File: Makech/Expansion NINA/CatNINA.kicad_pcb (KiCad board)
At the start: 2 copper layers, 22.9 x 30.9 mm, 10 parts, among them J1 ESP, U1 ESP32-WROOM

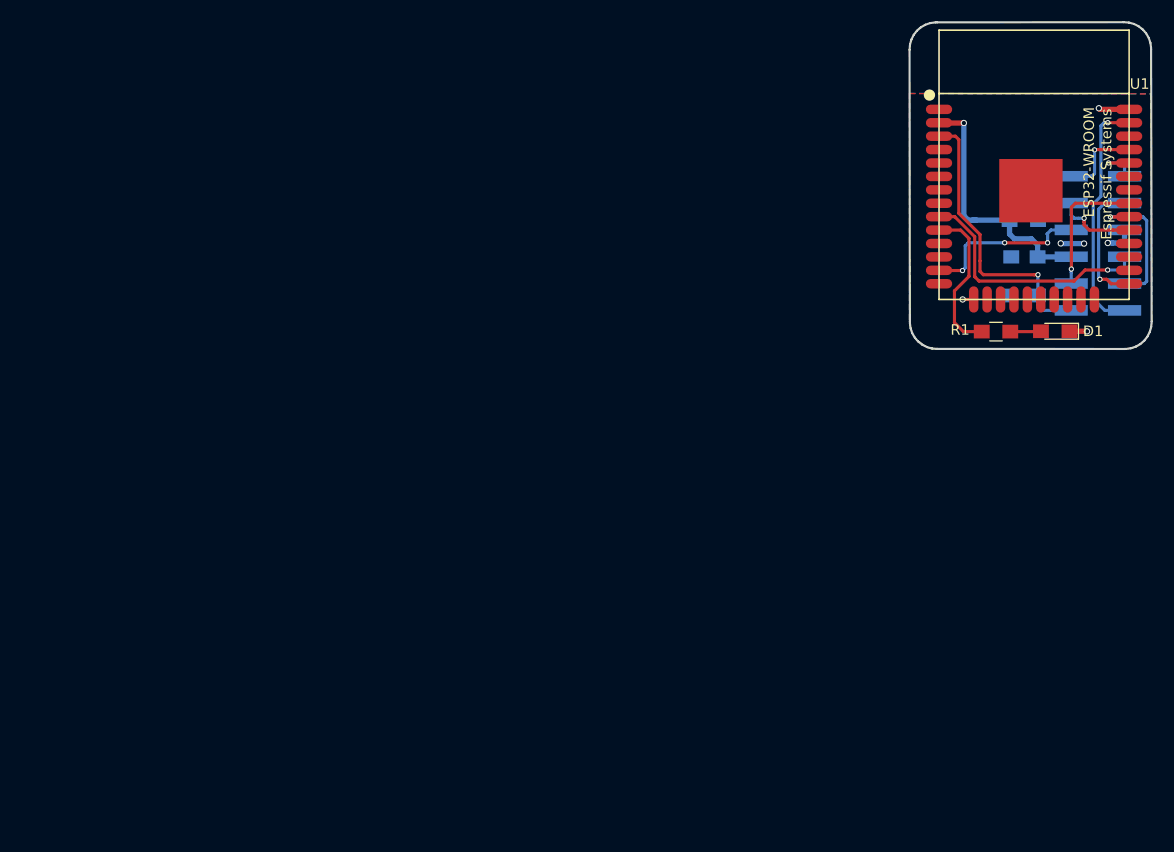
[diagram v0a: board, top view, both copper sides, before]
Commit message: mesures
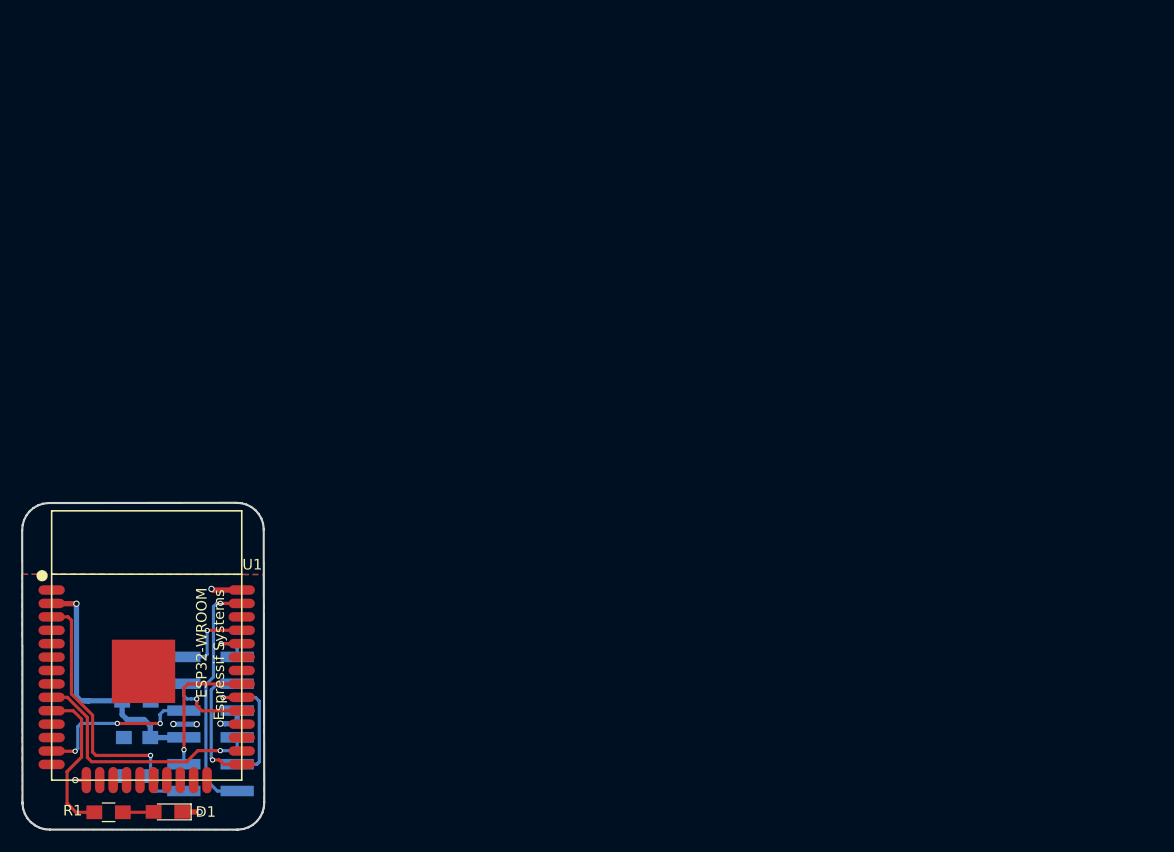
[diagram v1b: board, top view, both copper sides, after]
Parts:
- moved C1 95.6 mm to (160.2, 111.3)
- moved G*** 95.6 mm to (160.7, 101.5)
- moved D1 95.6 mm to (163.1, 118.3)
- moved G*** 95.6 mm to (153.8, 115.4)
- moved G*** 95.6 mm to (153.9, 103.2)
- moved R1 95.6 mm to (157.5, 118.4)
- moved R3 95.6 mm to (160.1, 107.8)
- moved J1 95.6 mm to (167.1, 110.0)
- moved R2 95.6 mm to (160.1, 115.0)
- moved U1 95.6 mm to (161.1, 102.6)
